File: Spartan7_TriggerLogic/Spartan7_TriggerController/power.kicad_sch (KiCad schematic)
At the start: 32 parts, among them U1 XC7S6-1FTGB196I

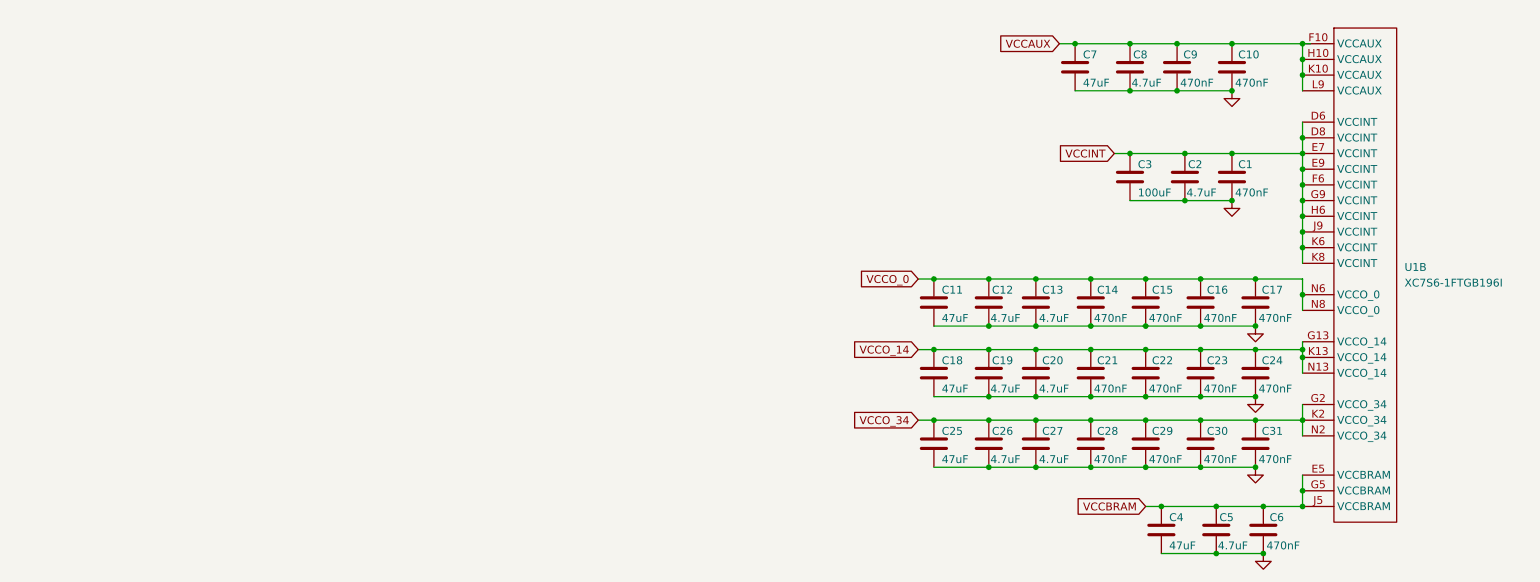
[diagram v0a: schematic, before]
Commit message: .
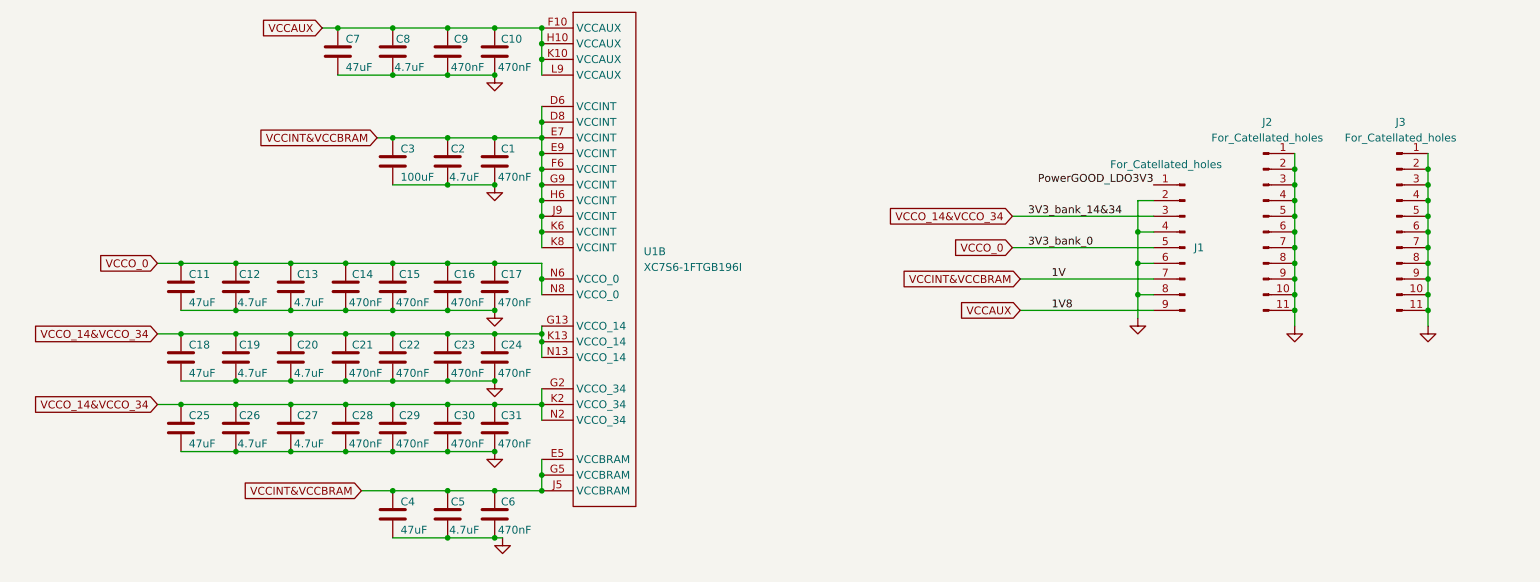
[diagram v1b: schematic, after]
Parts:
- added J1: For_Catellated_holes, Connector_PinHeader_2.54mm:PinHeader_1x09_P2.54mm_Vertical, symbol Connector:Conn_01x09_Pin
- added J2, J3: For_Catellated_holes, Connector_PinHeader_2.54mm:PinHeader_1x11_P2.54mm_Vertical, symbol Connector:Conn_01x11_Pin
- U1: footprint (none) -> 0_lib:BGA196C100P14X14_1500X1500X155N
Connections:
- net VCCINT is gone; now on net VCCINT&VCCBRAM: C1.1, C2.1, C3.1, U1.D6 (VCCINT), U1.D8 (VCCINT), U1.E7 (VCCINT), U1.E9 (VCCINT), U1.F6 (VCCINT), U1.G9 (VCCINT), U1.H6 (VCCINT), U1.J9 (VCCINT), U1.K6 (VCCINT), U1.K8 (VCCINT)
- net VCCO_34 is gone; now on net VCCO_14&VCCO_34: C25.1, C26.1, C27.1, C28.1, C29.1, C30.1, C31.1, U1.G2 (VCCO_34), U1.K2 (VCCO_34), U1.N2 (VCCO_34)
- net GND: now also J1.2 (Pin_2), J1.4 (Pin_4), J1.6 (Pin_6), J1.8 (Pin_8), J2.1 (Pin_1), J2.10 (Pin_10), J2.11 (Pin_11), J2.2 (Pin_2), J2.3 (Pin_3), J2.4 (Pin_4), J2.5 (Pin_5), J2.6 (Pin_6), J2.7 (Pin_7), J2.8 (Pin_8), J2.9 (Pin_9), J3.1 (Pin_1), J3.10 (Pin_10), J3.11 (Pin_11), J3.2 (Pin_2), J3.3 (Pin_3), J3.4 (Pin_4), J3.5 (Pin_5), J3.6 (Pin_6), J3.7 (Pin_7), J3.8 (Pin_8), J3.9 (Pin_9)
- net VCCAUX: now also J1.9 (Pin_9)
- net VCCO_0: now also J1.5 (Pin_5)
- net VCCBRAM renamed VCCINT&VCCBRAM
- net VCCINT&VCCBRAM: now also J1.7 (Pin_7)
- net VCCO_14 renamed VCCO_14&VCCO_34
- net VCCO_14&VCCO_34: now also J1.3 (Pin_3)
- new net PowerGOOD_LDO3V3: J1.1 (Pin_1)
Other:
- moved on the sheet: C1, C10, C11, C12, C13, C14, C15, C16, C17, C18, C19, C2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
